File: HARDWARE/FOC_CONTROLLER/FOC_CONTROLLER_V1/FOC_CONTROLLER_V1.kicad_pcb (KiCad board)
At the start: 2 copper layers, 34.3 x 34.3 mm, 98 parts, among them IC1 STSPIN32G0A2, IC2 MA330GQ-Z, J1 SM04B-GHS-TB_LF__SN_, J2 SM06B-GHS-TB_LF__SN_, Q1 DMT6018LDR-7, Q2 DMT6018LDR-7, Q3 DMT6018LDR-7

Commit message: up
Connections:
- IC1 pad 13: /UART_TX -> /MGH
- IC1 pad 14: /UART_RX -> /UART_TX
- IC1 pad 15: /MGL -> /UART_RX
- IC1 pad 16: /MGH -> /MGL
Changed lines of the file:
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@@
 			(size 0.3 0.85)
 			(layers "F.Cu" "F.Mask" "F.Paste")
-			(net 41 "/UART_TX")
+			(net 53 "/MGH")
 			(pinfunction "PA1")
 			(pintype "passive")
@@
 			(size 0.3 0.85)
 			(layers "F.Cu" "F.Mask" "F.Paste")
-			(net 49 "/UART_RX")
+			(net 41 "/UART_TX")
 			(pinfunction "PA2")
 			(pintype "passive")
@@
 			(size 0.3 0.85)
 			(layers "F.Cu" "F.Mask" "F.Paste")
-			(net 46 "/MGL")
+			(net 49 "/UART_RX")
 			(pinfunction "PA3")
 			(pintype "passive")
@@
 			(size 0.3 0.85)
 			(layers "F.Cu" "F.Mask" "F.Paste")
-			(net 53 "/MGH")
+			(net 46 "/MGL")
 			(pinfunction "PA4")
 			(pintype "passive")

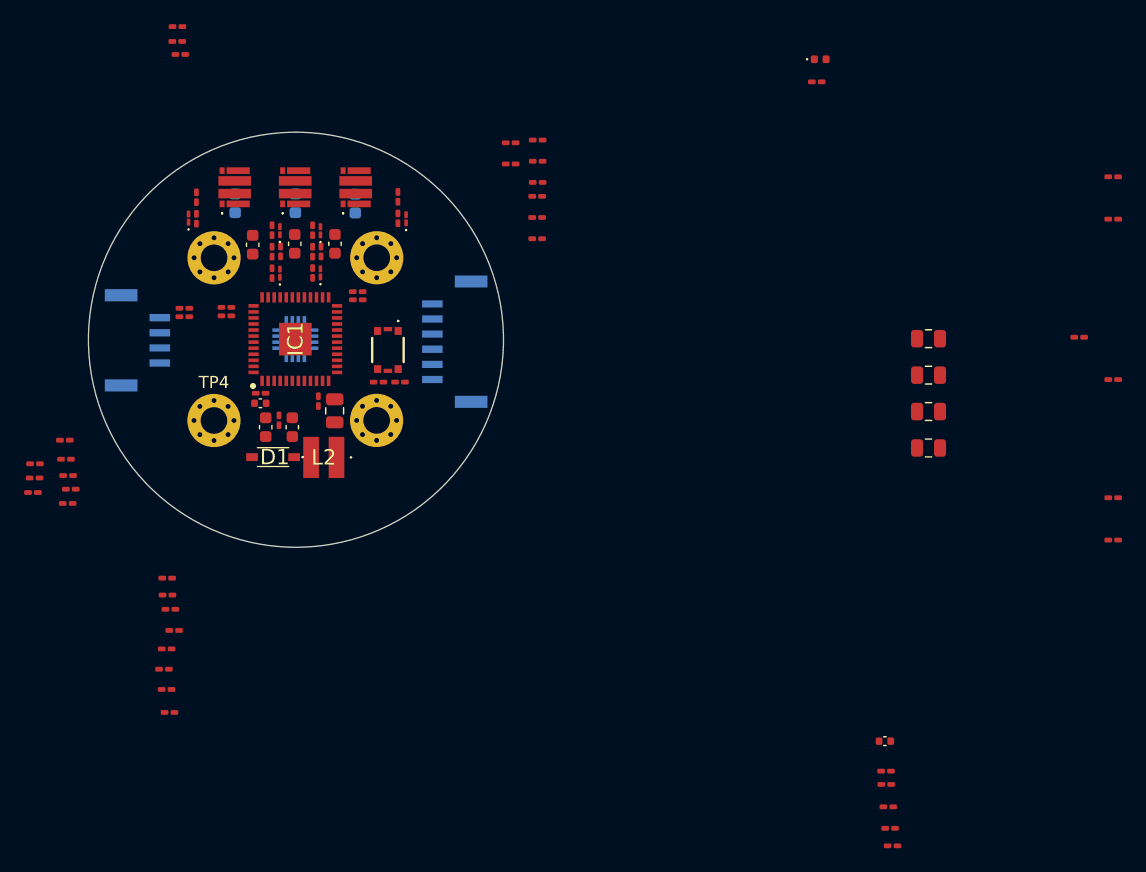
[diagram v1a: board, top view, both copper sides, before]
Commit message: update foc
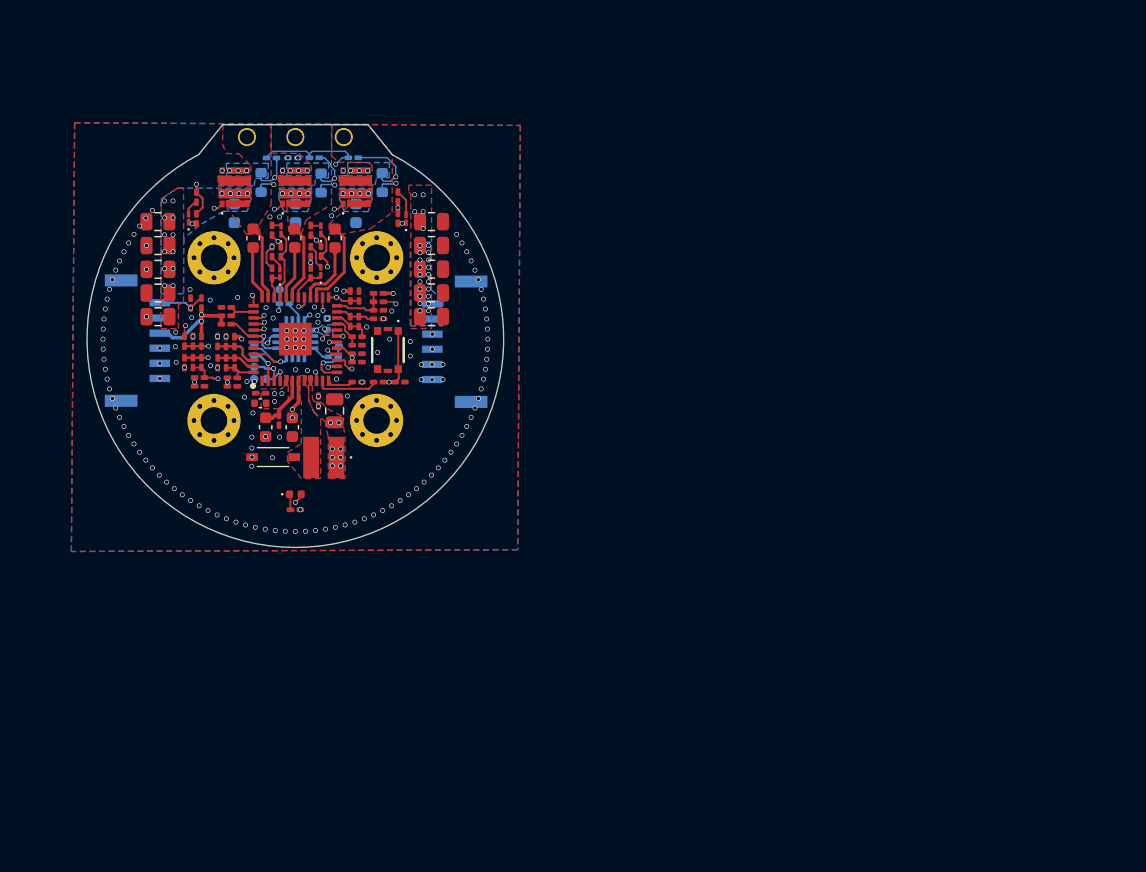
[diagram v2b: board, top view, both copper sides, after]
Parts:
- removed the C22 at (148.8, 135.7)
- removed R24, R35, R8: 10mR, Resistor_SMD:R_0201_0603Metric_Pad0.64x0.40mm_HandSolder
- added C23: 22u, Capacitor_SMD:C_0805_2012Metric, F.Cu at (88.7, 94.2)
- added C31: 22u, Capacitor_SMD:C_0805_2012Metric, F.Cu at (111.2, 94.2)
- added C33: 22u, Capacitor_SMD:C_0805_2012Metric, F.Cu at (88.7, 96.2)
- added C34: 22u, Capacitor_SMD:C_0805_2012Metric, F.Cu at (88.7, 98.2)
- added C35: 22u, Capacitor_SMD:C_0805_2012Metric, F.Cu at (111.2, 96.2)
- added C36: 22u, Capacitor_SMD:C_0805_2012Metric, F.Cu at (111.2, 98.1)
- added G***: LOGO, LOGO, F.Cu at (88.9, 106.5)
- added G***: LOGO, LOGO, F.Cu at (111.5, 106.5)
- added G***: LOGO, LOGO, B.Cu at (106.9, 111.3)
- added G***: LOGO, LOGO, B.Cu at (100.0, 113.3)
- added R48: R_Shunt, samacsys:4wire_0603, B.Cu at (97.2, 86.2)
- added R49: R_Shunt, samacsys:4wire_0603, B.Cu at (102.1, 86.3)
- added R50: R_Shunt, samacsys:4wire_0603, B.Cu at (107.2, 86.3)
- added TP10: TestPoint, samacsys:pad_0.7mm, B.Cu at (96.6, 101.4)
- added TP11: TestPoint, samacsys:pad_0.7mm, B.Cu at (98.7, 95.9)
- added TP12: TestPoint, samacsys:pad_0.7mm, B.Cu at (103.6, 100.6)
- added TP13: TestPoint, samacsys:pad_0.7mm, B.Cu at (96.6, 100.5)
- added TP15: TestPoint, samacsys:pad_0.7mm, B.Cu at (96.6, 103.3)
- added TP5: TestPoint, samacsys:hole_1.5mm, F.Cu at (96.0, 83.3)
- added TP6: TestPoint, samacsys:hole_1.5mm, F.Cu at (100.0, 83.3)
- added TP7: TestPoint, samacsys:hole_1.5mm, F.Cu at (104.0, 83.3)
- added TP8: TestPoint, samacsys:pad_0.7mm, B.Cu at (97.6, 103.3)
- added TP9: TestPoint, samacsys:pad_0.7mm, B.Cu at (96.6, 102.3)
- C22, R38, R39, R41, R43, R44, R45: moved to B.Cu
- C24, C25, C26, C27: value 47u -> 22u
- C8: value 100n -> 10n
- J1: value SM04B-GHS-TB_LF__SN_ -> SM06B-GHS-TB_LF__SN_; footprint samacsys:SM04B-GHS-TB -> samacsys:SM06B-GHS-TB
- moved R43 71.9 mm to (98.0, 85.0), turned to 180 degrees
- moved R45 70.3 mm to (104.8, 85.0), turned to 180 degrees
- moved R1 66.5 mm to (94.3, 98.8), turned to 180 degrees
- moved C27 66.4 mm to (88.6, 90.3), turned to 180 degrees
- moved R38 66.2 mm to (99.1, 97.1)
- moved R44 66.2 mm to (101.6, 85.0), turned to 180 degrees
- moved C26 65.1 mm to (88.7, 92.3), turned to 180 degrees
- moved R39 61.4 mm to (103.1, 101.5)
- moved C22 57.6 mm to (102.6, 98.8), turned to 90 degrees
- moved D8 56.3 mm to (100.0, 112.8)
- moved R37 56.2 mm to (105.1, 103.5)
- moved R47 55.7 mm to (100.0, 114.1), turned to 180 degrees
- moved C25 42.4 mm to (111.2, 92.3)
- moved C24 42.2 mm to (111.2, 90.3)
- moved C29 30.8 mm to (105.1, 101.2)
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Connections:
- C15 pad 2: /ISNSU -> /ISNSW
- C18 pad 2: /ISNSV -> /ISNSU
- C21 pad 2: /ISNSW -> /ISNSV
- C9 pad 1: Net-(S1-NO_1) -> /NRST
- IC1 pad 18: /ISNSU -> /ISNSV
- IC1 pad 20: /ISNSV -> /ISNSU
- J1 pad 1: /SWCLK -> /NRST
- J1 pad 2: /SWDIO -> /SWCLK
- J1 pad 3: GND -> /SWDIO
- J1 pad 4: /BTN -> +3.3V
- J1 pad 5: (no net) -> GND
- J1 pad 6: (no net) -> /BTN
- J2 pad 7: (no net) -> GND
- J2 pad 8: (no net) -> GND
- Q1 pad 3: /U/SHUNT+ -> Net-(Q1-S2)
- Q2 pad 3: /V/SHUNT+ -> Net-(Q2-S2)
- Q3 pad 3: /W/SHUNT+ -> Net-(Q3-S2)
- R10 pad 1: /U/SHUNT+ -> /SHUNT+W
- R14 pad 2: /ISNSU -> /ISNSW
- R15 pad 1: /V/SHUNT+ -> /SHUNT+U
- R22 pad 1: GND -> /SHUNT-U
- R25 pad 2: /ISNSV -> /ISNSU
- R26 pad 1: /W/SHUNT+ -> /SHUNT+V
- R3 pad 2: Net-(S1-NO_1) -> /NRST
- R33 pad 1: GND -> /SHUNT-V
- R36 pad 2: /ISNSW -> /ISNSV
- R43 pad 1: /U/SHUNT+ -> /SHUNT+U
- R44 pad 1: /V/SHUNT+ -> /SHUNT+V
- R45 pad 1: /W/SHUNT+ -> /SHUNT+W
- R9 pad 1: GND -> /SHUNT-W
- S1 pad 1: Net-(S1-NO_1) -> /NRST
- S1 pad 2: Net-(S1-NO_1) -> /NRST
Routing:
- net Net-(IC1-PA5): track 0.00 -> 27.0 mm, vias 0 -> 2
- net +3.3V: track 0.00 -> 24.9 mm, vias 0 -> 20
- net /NRST: track 0.00 -> 24.9 mm, vias 0 -> 2
- net /SHUNT+AFTER: track 0.00 -> 24.3 mm, vias 0 -> 2
- net /SHUNT+V: track 0.00 -> 21.6 mm, vias 0 -> 2
- net /SHUNT+U: track 0.00 -> 20.7 mm, vias 0 -> 2
- net /SHUNT-V: track 0.00 -> 20.6 mm, vias 0 -> 2
- net /SHUNT-U: track 0.00 -> 19.7 mm, vias 0 -> 2
- net /SHUNT+W: track 0.00 -> 19.0 mm, vias 0 -> 2
- net /SHUNT-W: track 0.00 -> 14.9 mm, vias 0 -> 2
- net /ISNSU: track 0.00 -> 14.7 mm, vias 0 -> 2
- net /HSW: track 0.00 -> 13.7 mm, vias 0 -> 2
- net Net-(D8-A): track 0.00 -> 13.1 mm, vias 0 -> 2
- net /ISNSV: track 0.00 -> 11.6 mm, vias 0 -> 2
- net /LSU: track 0.00 -> 11.3 mm, vias 0 -> 2
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- added copper zone on B.Cu, net +3.3V
- added copper zone on F.Cu, net +3.3V
- added copper zone on In4.Cu, net +3.3V
- added copper zone on F.Cu, net /OUTU
- added copper zone on F.Cu, net /OUTV
- added copper zone on F.Cu, net /OUTW
- added copper zone on F.Cu, net /SW
- added copper zone on B.Cu, net GND
- added copper zone on F.Cu, net GND
- added copper zone on In1.Cu, net GND
- added copper zone on In2.Cu, net GND
- added copper zone on In3.Cu, net GND
- added copper zone on In4.Cu, net GND
- added copper zone on In6.Cu, net GND
- added copper zone on B.Cu, net Net-(Q1-S2)
- added copper zone on B.Cu, net Net-(Q2-S2)
- added copper zone on B.Cu, net Net-(Q3-S2)
- added copper zone on B.Cu, net VBAT+
- added copper zone on F.Cu, net VBAT+
- added copper zone on In5.Cu, net VBAT+
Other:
- board size 34.3 x 34.3 mm -> 34.4 x 34.9 mm
- copper layers 2 -> 8
- board text added: "3.3V"
- board text added: "BTN"
- board text added: "GND"
- board text added: "LED"
- board text added: "MGH"
- board text added: "MGL"
- board text added: "NRST"
- board text added: "OP2N"
- board text added: "OP2O"
- board text added: "OP2P"
- board text added: "RX"
- board text added: "SPI2_MOSI"
- board text added: "SWCLK"
- board text added: "SWDIO"
- board text added: "TX"
- board text added: "VBAT+"
